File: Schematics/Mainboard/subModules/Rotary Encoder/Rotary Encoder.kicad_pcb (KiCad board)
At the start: 2 copper layers, 22.1 x 22.1 mm, 7 parts, among them J1 Power, J2 Data, SW1 Rot

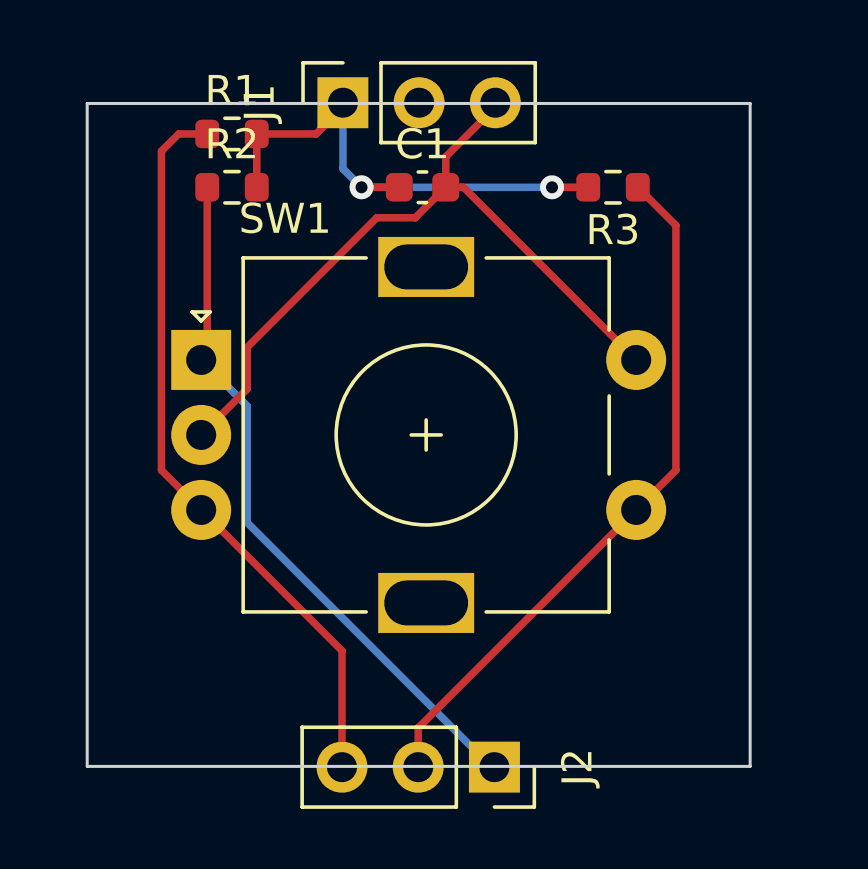
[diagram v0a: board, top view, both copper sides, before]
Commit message: Moved F.Fab
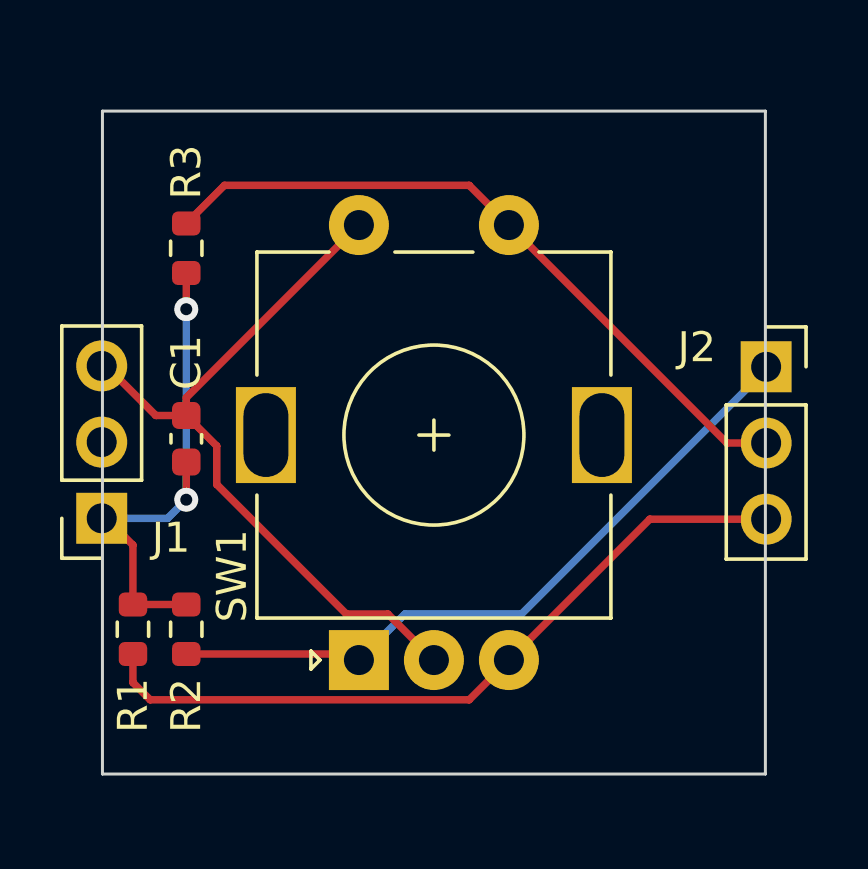
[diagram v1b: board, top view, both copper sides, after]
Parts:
- moved R1 16.8 mm to (134.6, 107.7), turned to 90 degrees
- moved J2 16.1 mm to (155.7, 98.9), turned to 0 degrees
- moved J1 16.0 mm to (133.6, 104.0), turned to 180 degrees
- moved R2 14.8 mm to (136.4, 107.7), turned to 90 degrees
- moved R3 14.4 mm to (136.4, 95.0), turned to -90 degrees
- moved C1 11.5 mm to (136.4, 101.3), turned to 90 degrees
- moved SW1 11.3 mm to (142.2, 108.7), turned to 90 degrees
